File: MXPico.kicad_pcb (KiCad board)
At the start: 2 copper layers, 117.5 x 76.8 mm, 28 parts, among them J1 JST PH 4-pin, J2 JST PH 4-pin, J3 Conn_02x17_Odd_Even, U1 Pico

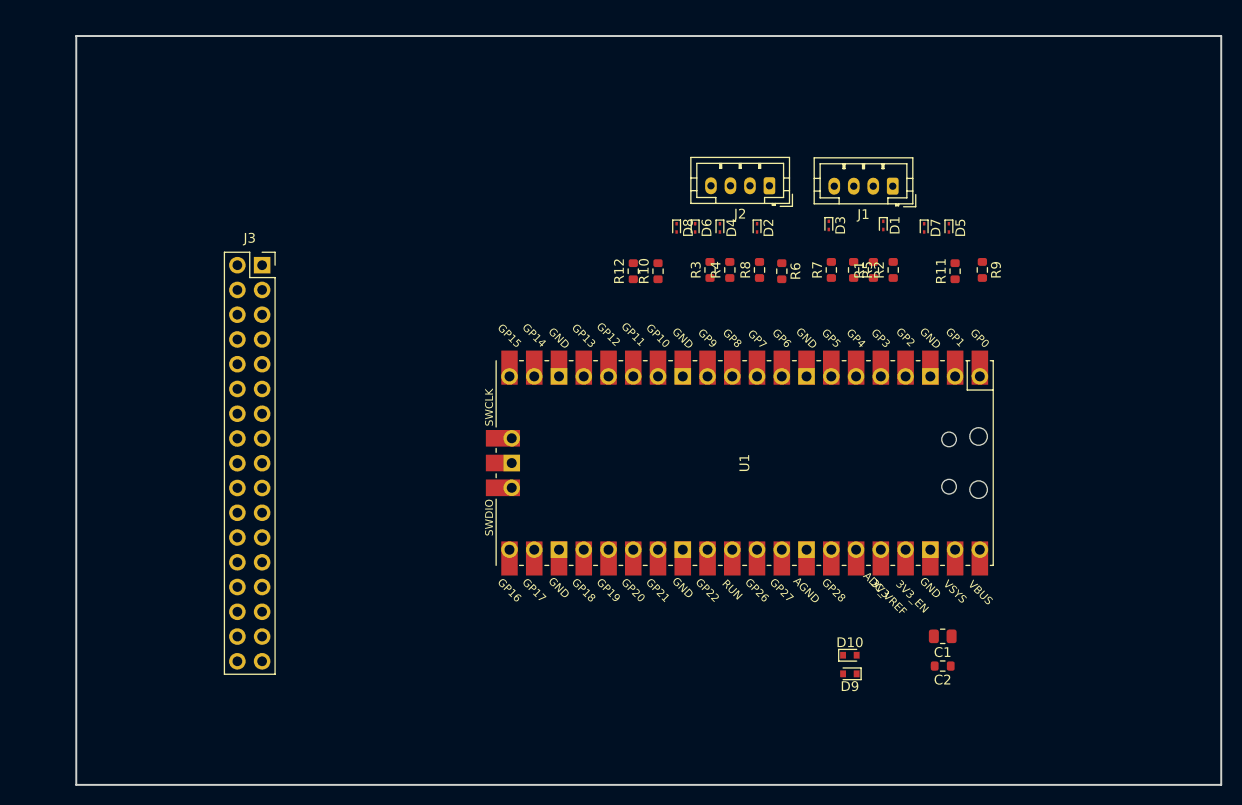
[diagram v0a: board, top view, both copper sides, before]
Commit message: Adds initial layout and fab files for E1
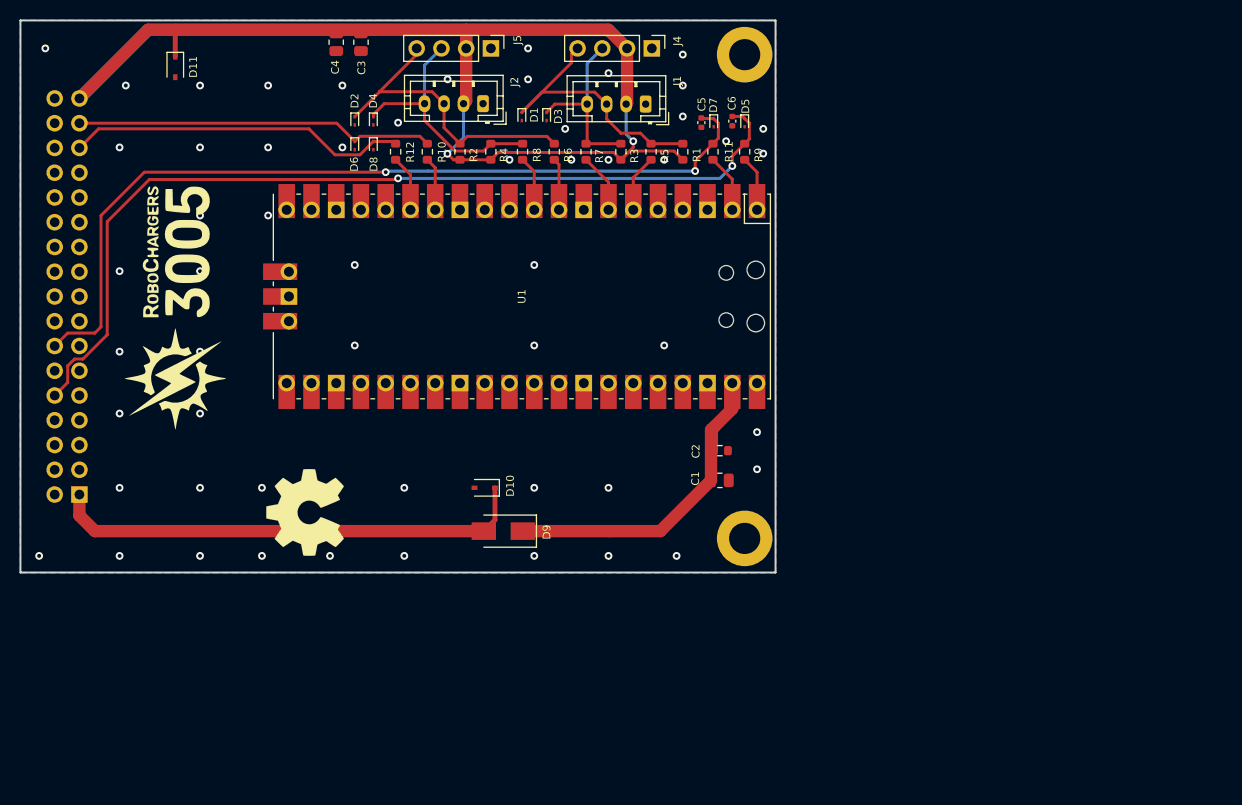
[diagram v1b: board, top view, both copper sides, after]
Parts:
- added C3: 10uF, Resistor_SMD:R_0805_2012Metric, F.Cu at (114.9, 62.2)
- added C4: 10uF, Resistor_SMD:R_0805_2012Metric, F.Cu at (112.4, 62.2)
- added C5: 100pF, Capacitor_SMD:C_0402_1005Metric, F.Cu at (149.9, 70.5)
- added C6: 100pF, Capacitor_SMD:C_0402_1005Metric, F.Cu at (153.0, 70.3)
- added D11: TVS, Diode_SMD:D_SOD-323, F.Cu at (95.9, 64.8)
- added G***: LOGO, RoboChargers:RoboChargers, F.Cu at (95.9, 89.5)
- added H1: MountingHole, MountingHole:MountingHole_3.2mm_M3_ISO7380_Pad, F.Cu at (154.3, 63.5)
- added H2: MountingHole, MountingHole:MountingHole_3.2mm_M3_ISO7380_Pad, F.Cu at (154.3, 113.1)
- added J4: 100mil Header, Connector_PinHeader_2.54mm:PinHeader_1x04_P2.54mm_Vertical, F.Cu at (144.8, 62.9)
- added J5: 100mil Header, Connector_PinHeader_2.54mm:PinHeader_1x04_P2.54mm_Vertical, F.Cu at (128.3, 62.9)
- added REF**: OSHW-Symbol_8.9x8mm_SilkScreen, Symbol:OSHW-Symbol_8.9x8mm_SilkScreen, F.Cu at (109.2, 110.5)
- D10: value D_Zener -> TVS; footprint Diode_SMD:D_SOD-523 -> Diode_SMD:D_SOD-323
- D9: footprint Diode_SMD:D_SOD-523 -> Diode_SMD:D_SMA
- J3: value Conn_02x17_Odd_Even -> SH2-34G-P; moved to B.Cu
- moved R2 46.1 mm to (125.1, 73.5)
- moved D2 42.7 mm to (114.3, 70.3)
- moved D10 41.2 mm to (127.6, 108.0), turned to 180 degrees
- moved D1 38.7 mm to (131.4, 69.8)
- moved D9 38.5 mm to (129.5, 112.4)
- moved D4 37.2 mm to (116.2, 70.3)
- moved D6 35.9 mm to (114.3, 72.8)
- moved D8 32.2 mm to (116.2, 72.8)
- moved C2 31.8 mm to (151.8, 104.1), turned to 0 degrees
- moved D3 31.0 mm to (134.0, 69.8)
- moved J2 30.6 mm to (127.5, 68.5)
- moved J3 30.1 mm to (86.0, 108.6)
- moved U1 28.5 mm to (131.4, 88.3)
- moved R7 27.9 mm to (138.0, 73.5)
- moved C1 27.9 mm to (151.8, 107.2), turned to 0 degrees
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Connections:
- J3 pad 18: /PULSE0 -> unconnected-(J3-Pad18)
- J3 pad 22: /PULSE1 -> unconnected-(J3-Pad22)
- J3 pad 29: unconnected-(J3-Pad29) -> /PULSE1
- J3 pad 31: unconnected-(J3-Pad31) -> /PULSE0
- J3 pad 33: unconnected-(J3-Pad33) -> +3V3
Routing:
- net +3V3: track 0.00 -> 176.4 mm, vias 0 -> 2
- net /PICO_TX: track 0.00 -> 94.2 mm, vias 0 -> 2
- net /PICO_RX: track 0.00 -> 87.8 mm, vias 0 -> 2
- net +5V: track 0.00 -> 49.2 mm
- net /PULSE0: track 0.00 -> 37.0 mm
- net /PULSE1: track 0.00 -> 35.0 mm
- net Net-(C1-Pad1): track 0.00 -> 34.7 mm
- net Net-(D2-Pad1): track 0.00 -> 31.8 mm
- net Net-(D1-Pad1): track 0.00 -> 29.4 mm
- net Net-(D4-Pad1): track 0.00 -> 25.7 mm
- net Net-(D3-Pad1): track 0.00 -> 18.6 mm
- net /SCL0: track 0.00 -> 6.09 mm
- net /SDA1: track 0.00 -> 6.02 mm
- net Net-(R11-Pad1): track 0.00 -> 5.96 mm
- net /SDA0: track 0.00 -> 5.89 mm
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- added copper zone on B.Cu, net GND
- added copper zone on F.Cu, net GND
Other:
- board size 117.5 x 76.8 mm -> 77.5 x 56.6 mm
- board text added: "2022-E1"
